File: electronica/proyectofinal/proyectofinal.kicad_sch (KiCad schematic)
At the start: 16 parts, among them J1 cnn, J2 conector alimentacion esp, J3 dht22, J4 Guva-s12s, J5 convertidor_TTL, J6 MICS-6814, K1 SRD-05VDC-SL-C, K2 SRD-05VDC-SL-C, U1 LM7833_TO220, U3 LM7805_TO220, U4 ESP32_LORA_V2.0

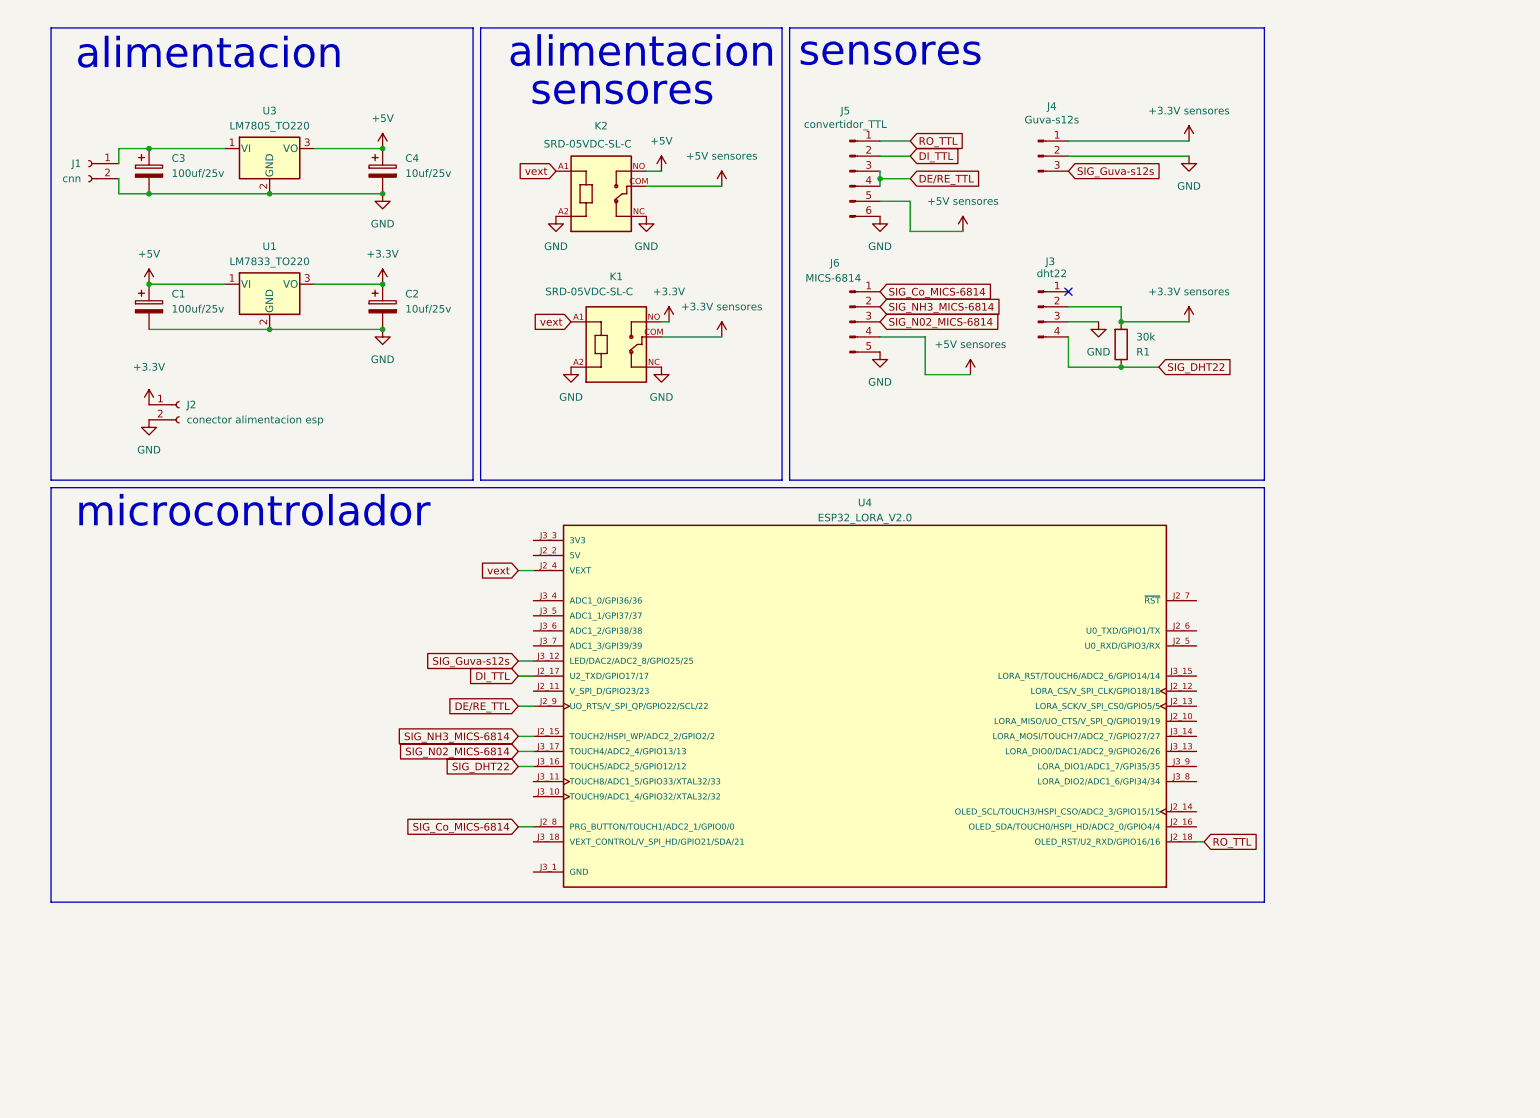
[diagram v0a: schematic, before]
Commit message: loisto
st
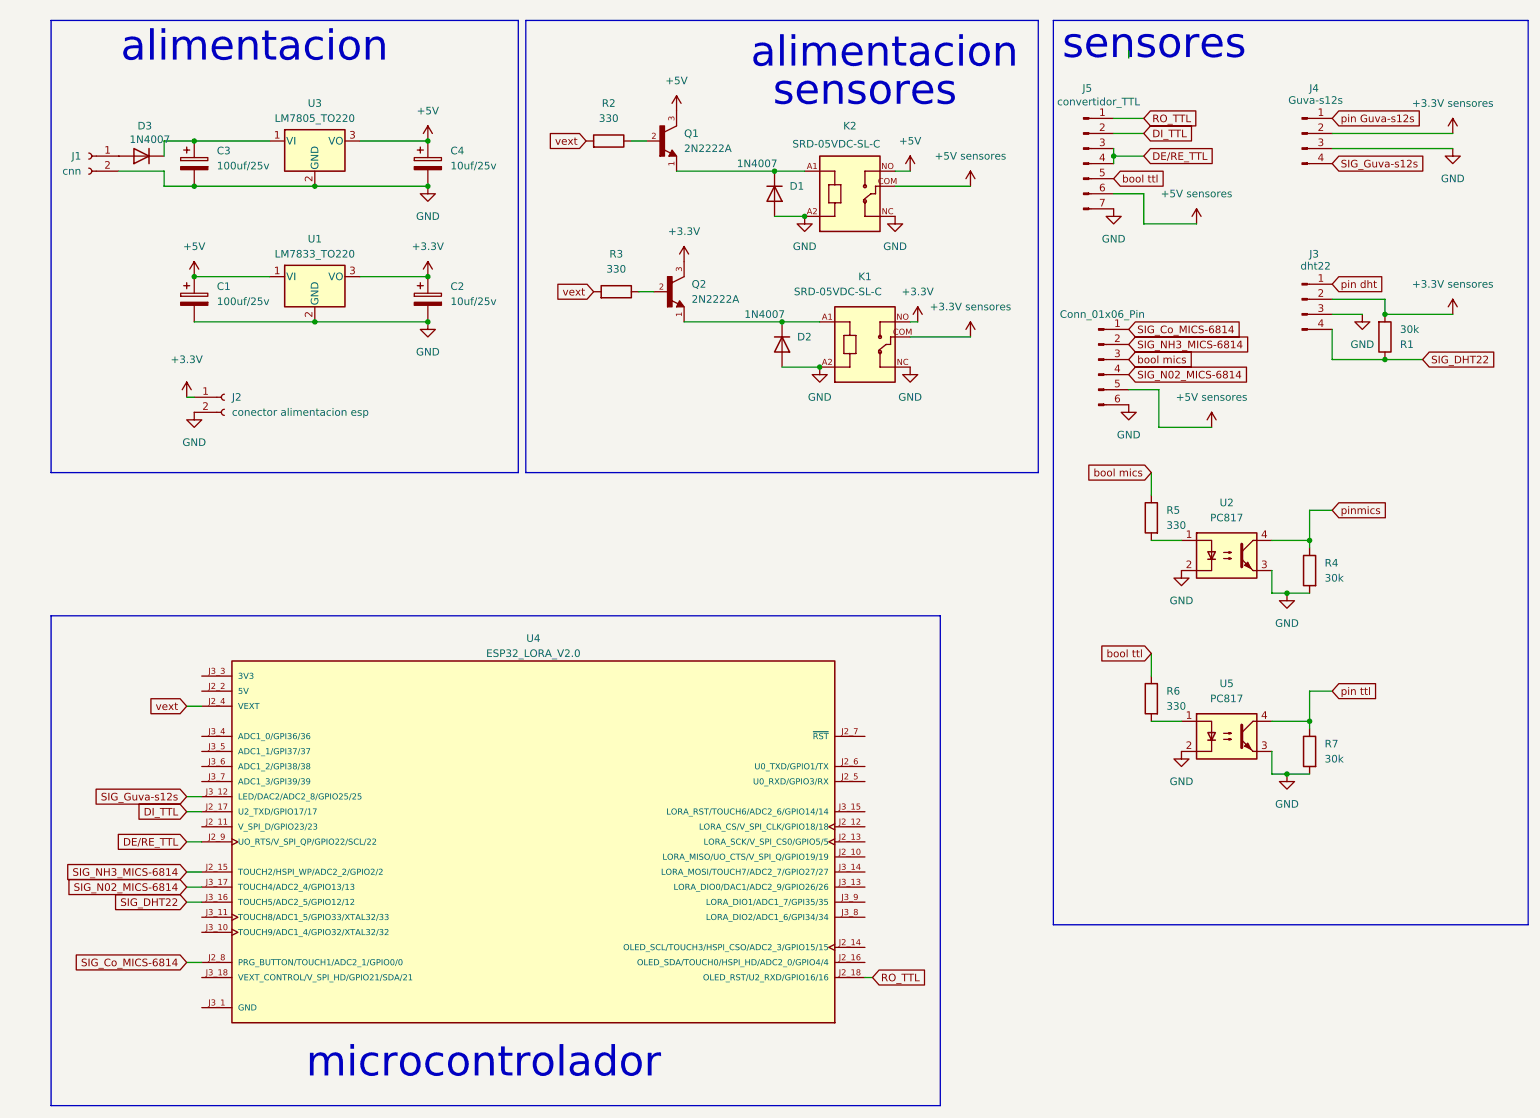
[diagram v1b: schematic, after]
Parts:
- removed J4: Guva-s12s, Connector_Molex:Molex_KK-254_AE-6410-03A_1x03_P2.54mm_Vertical, symbol Connector:Conn_01x03_Pin
- removed J5: convertidor_TTL, Connector_Molex:Molex_KK-254_AE-6410-06A_1x06_P2.54mm_Vertical, symbol Connector:Conn_01x06_Pin
- removed J6: MICS-6814, Connector_Molex:Molex_KK-254_AE-6410-05A_1x05_P2.54mm_Vertical, symbol Connector:Conn_01x05_Pin
- added D1, D2, D3: 1N4007, Diode_THT:D_DO-41_SOD81_P10.16mm_Horizontal, symbol Diode:1N4007
- added J4: Guva-s12s, Connector_Molex:Molex_KK-254_AE-6410-04A_1x04_P2.54mm_Vertical, symbol Connector:Conn_01x04_Pin
- added J5: convertidor_TTL, Connector_Molex:Molex_KK-254_AE-6410-07A_1x07_P2.54mm_Vertical, symbol Connector:Conn_01x07_Pin
- added J7: Conn_01x06_Pin, Connector_Molex:Molex_KK-254_AE-6410-06A_1x06_P2.54mm_Vertical, symbol Connector:Conn_01x06_Pin
- added Q1, Q2: 2N2222A, 2N2222A:TO92254P470H750-3, symbol 2N2222A:2N2222A
- added R2, R3, R5, R6: 330, Resistor_THT:R_Axial_DIN0207_L6.3mm_D2.5mm_P10.16mm_Horizontal, symbol Device:R
- added R4, R7: 30k, Resistor_THT:R_Axial_DIN0207_L6.3mm_D2.5mm_P10.16mm_Horizontal, symbol Device:R
- added U2, U5: PC817, Package_DIP:DIP-4_W7.62mm, symbol Isolator:PC817
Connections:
- net +3.3V: now also Q2.3
- net +3.3V sensores: now also J4.2 (Pin_2)
- net +5V: now also Q1.3
- net +5V sensores: now also J5.6 (Pin_6), J7.5 (Pin_5)
- net DE/RE_TTL: now also J5.3 (Pin_3), J5.4 (Pin_4)
- net DI_TTL: now also J5.2 (Pin_2)
- net GND: now also D1.2 (A), D2.2 (A), J4.3 (Pin_3), J5.7 (Pin_7), J7.6 (Pin_6), R4.2, R7.2, U2.2, U2.3, U5.2, U5.3
- net RO_TTL: now also J5.1 (Pin_1)
- net SIG_Co_MICS-6814: now also J7.1 (Pin_1)
- net SIG_Guva-s12s: now also J4.4 (Pin_4)
- net SIG_N02_MICS-6814: now also J7.4 (Pin_4)
- net SIG_NH3_MICS-6814: now also J7.2 (Pin_2)
- net vext: now also R2.2, R3.2; no longer K1.A1, K2.A1
- net at C3.1, U3.1 (VI): now also D3.1 (K); no longer J1.1 (Pin_1)
- net pin dht: now reaches J3.1 (Pin_1)
- new net: Q2.2, R3.1
- new net: D2.1 (K), K1.A1, Q2.1
- new net: R6.2, U5.1
- new net: R5.2, U2.1
- new net: D3.2 (A), J1.1 (Pin_1)
- new net: D1.1 (K), K2.A1, Q1.1
- new net: Q1.2, R2.1
- new net bool mics: J7.3 (Pin_3), R5.1
- new net bool ttl: J5.5 (Pin_5), R6.1
- new net pin Guva-s12s: J4.1 (Pin_1)
- new net pin ttl: R7.1, U5.4
- new net pinmics: R4.1, U2.4
- no-connect marks 1 -> 0
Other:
- moved on the sheet: C1, C2, C3, C4, J1, J2, J3, K1, K2, R1, U1, U3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
